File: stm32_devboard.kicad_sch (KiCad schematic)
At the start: 39 parts, among them J1 Conn_01x04_Male, J2 USB_B_Micro, SW1 SW_SPDT, U2 STM32F103CBT6, Y1 Crystal_GND24

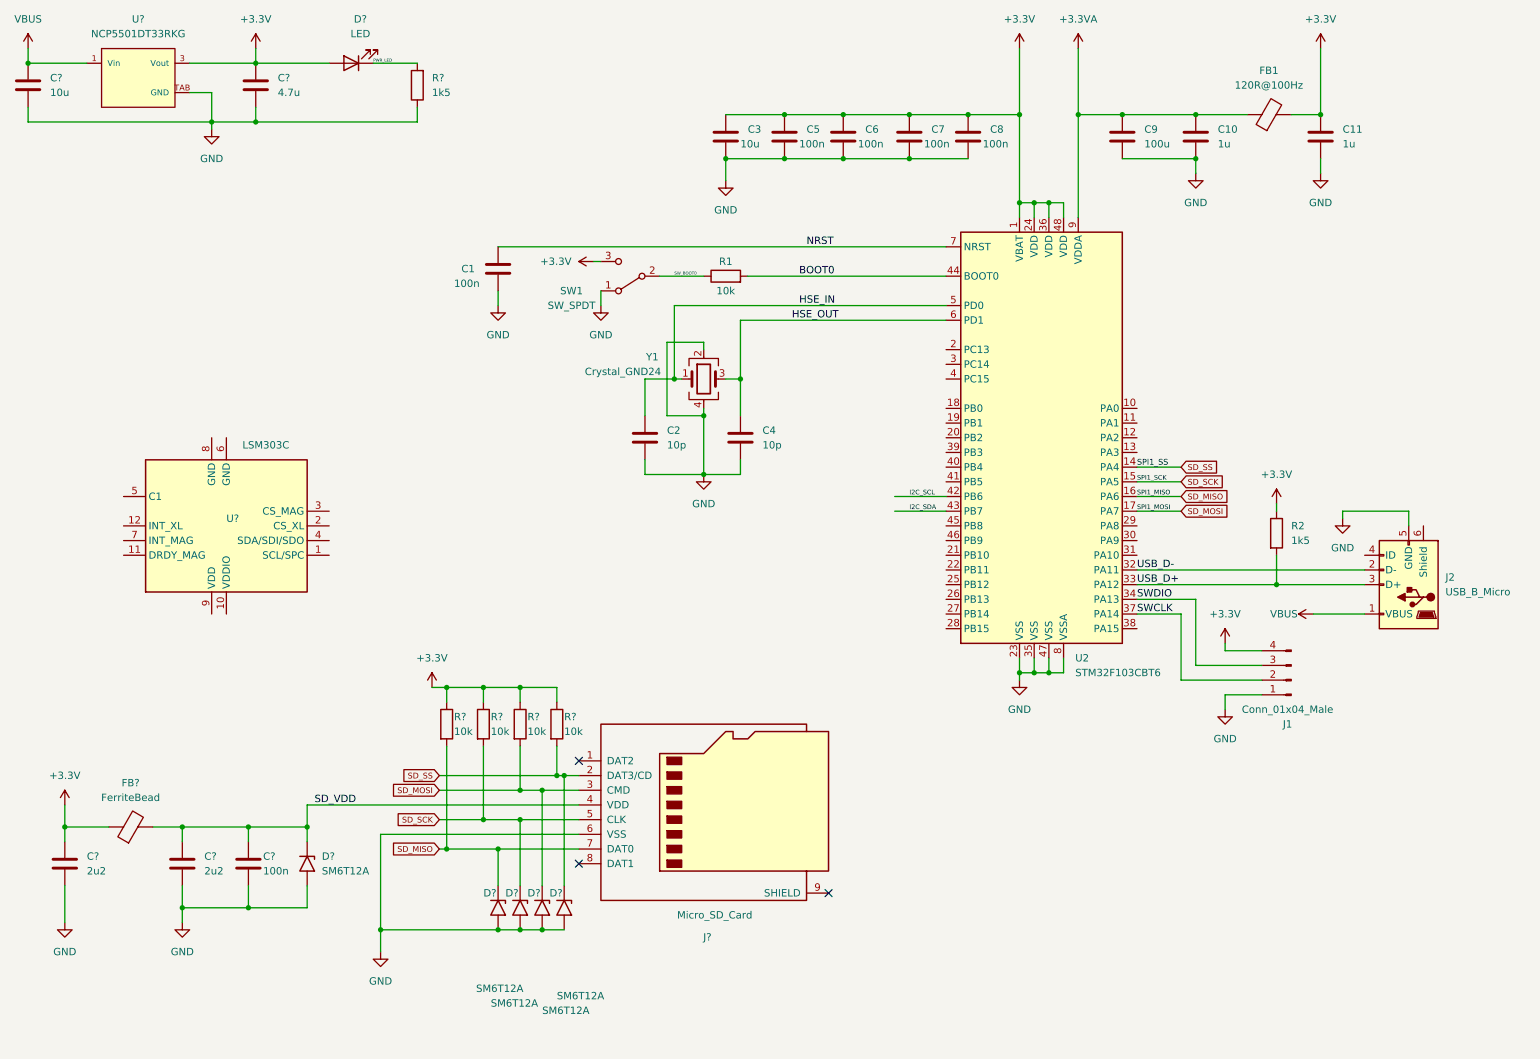
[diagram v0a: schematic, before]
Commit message: add imu
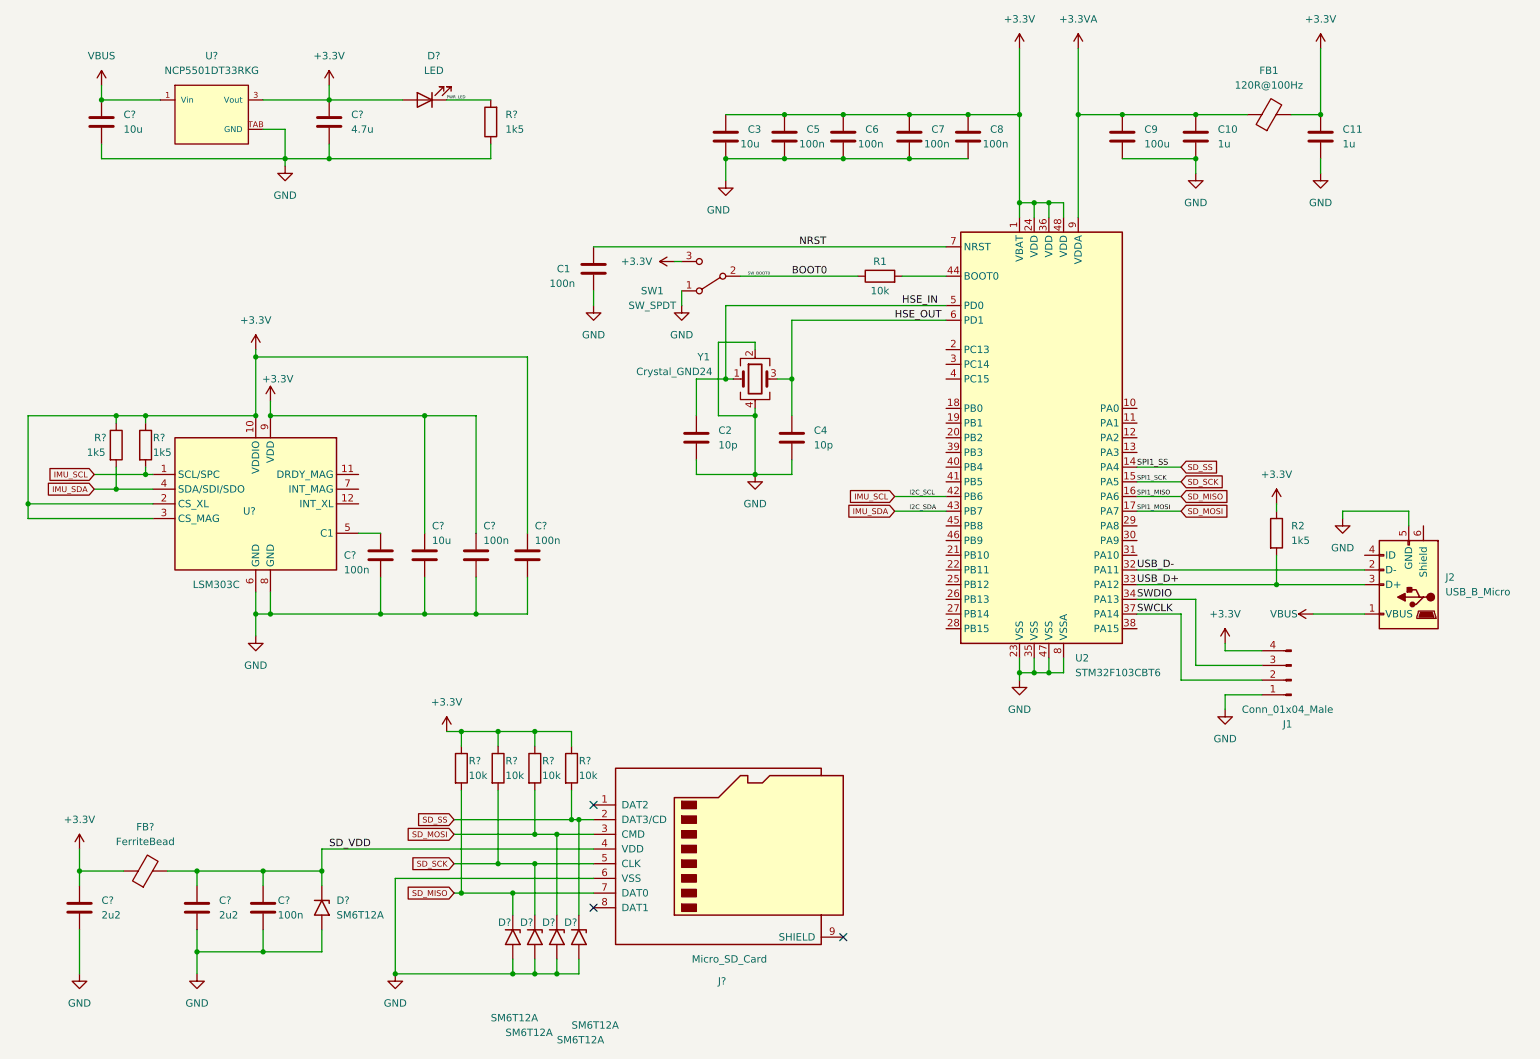
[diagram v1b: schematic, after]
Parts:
- added C? (x3): 100n, symbol Device:C
- added C?: 10u, symbol Device:C
- added R? (x2): 1k5, symbol Device:R
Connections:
- net I2C_SCL is gone; now on net IMU_SCL: U2.42 (PB6)
- net I2C_SDA is gone; now on net IMU_SDA: U2.43 (PB7)
- net SW_BOOT0 is gone; now on net BOOT0: R1.1, SW1.2 (B)
- net +3V3: now also U?.10 (VDDIO), U?.2 (CS_XL), U?.3 (CS_MAG), U?.9 (VDD), C?.1, C?.1, C?.1, R?.1, R?.1
- net BOOT0: no longer R1.2, U2.44 (BOOT0)
- net GND: now also U?.6 (GND), U?.8 (GND), C?.2, C?.2, C?.2, C?.2
- net IMU_SCL: now reaches U?.1 (SCL/SPC)
- net IMU_SCL: now also R?.2
- net IMU_SDA: now reaches U?.4 (SDA/SDI/SDO)
- net IMU_SDA: now also R?.2
- net at U?.5 (C1): now also C?.1
- new net: R1.2, U2.44 (BOOT0)
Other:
- moved on the sheet: C1, C2, C4, C?, D?, FB?, J?, R1, R?, SW1, U?, Y1
